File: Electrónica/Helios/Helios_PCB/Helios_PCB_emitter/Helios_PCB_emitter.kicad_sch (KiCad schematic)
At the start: 8 parts, among them J1 Conn_01x03_Male, Q0 AO3400A

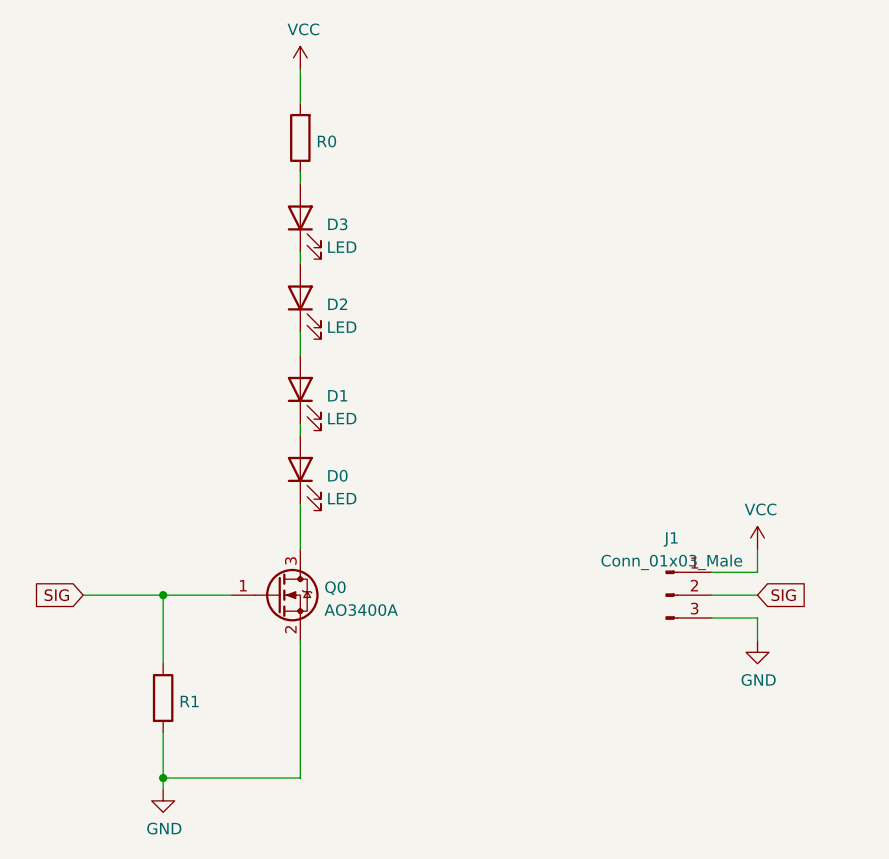
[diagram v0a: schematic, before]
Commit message: Helios Panel
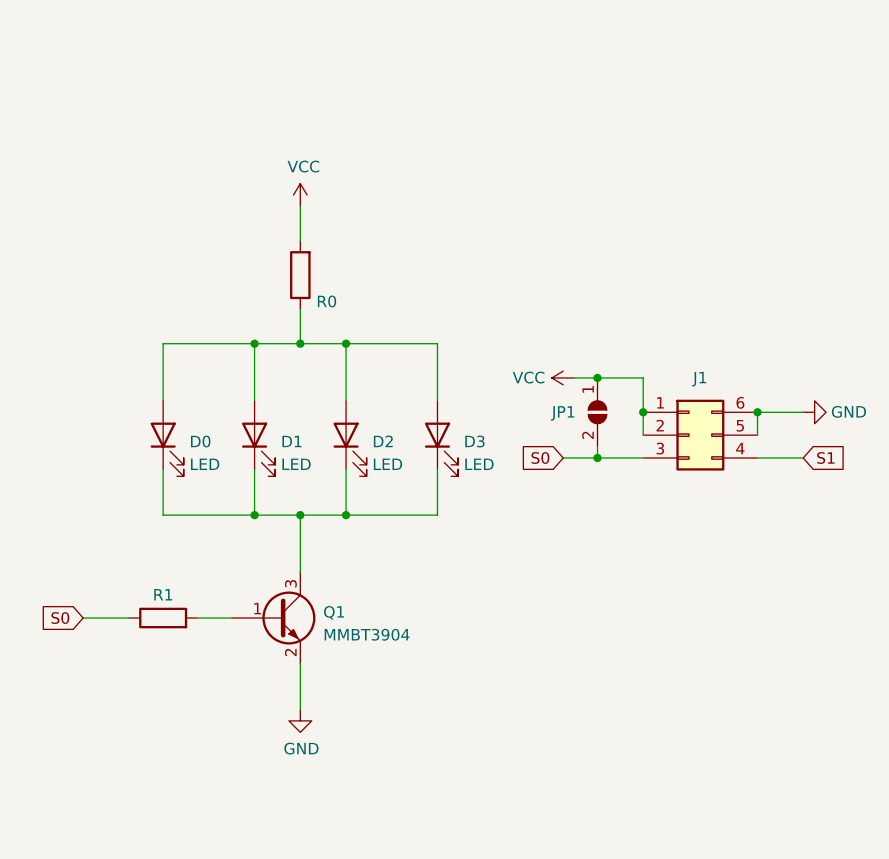
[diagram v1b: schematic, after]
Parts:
- removed J1: Conn_01x03_Male, Connector_PinHeader_2.54mm:PinHeader_1x03_P2.54mm_Vertical, symbol Connector:Conn_01x03_Male
- removed Q0: AO3400A, Package_TO_SOT_SMD:SOT-23, symbol Transistor_FET:AO3400A
- added J1: Conn_02x03_Counter_Clockwise, Connector_PinHeader_2.54mm:PinHeader_2x03_P2.54mm_Vertical, symbol Connector_Generic:Conn_02x03_Counter_Clockwise
- added JP1: SolderJumper_2_Open, Jumper:SolderJumper-2_P1.3mm_Open_Pad1.0x1.5mm, symbol Jumper:SolderJumper_2_Open
- added Q1: MMBT3904, Package_TO_SOT_SMD:SOT-23, symbol Transistor_BJT:MMBT3904
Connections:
- net GND: now also J1.5 (Pin_5), J1.6 (Pin_6), Q1.2 (E); no longer R1.2
- net VCC: now also J1.1 (Pin_1), J1.2 (Pin_2), JP1.1 (A)
- net at D1.1 (K): now also D0.1 (K), D2.1 (K), D3.1 (K), Q1.3 (C); no longer D0.2 (A)
- net at D1.2 (A): now also D0.2 (A), D2.2 (A), D3.2 (A), R0.1; no longer D2.1 (K)
- net SIG renamed S0
- net S0: now also J1.3 (Pin_3), JP1.2 (B)
- new net: Q1.1 (B), R1.2
- new net S1: J1.4 (Pin_4)
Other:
- moved on the sheet: D0, D1, D2, D3, R0, R1
